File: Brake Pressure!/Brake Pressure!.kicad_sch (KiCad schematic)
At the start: 12 parts, among them J1 DTF13-6P, Q1 Q_Photo_NPN_EBC, U1 TJA1050DRG, U2 MCP2515-I, X1 ${ALTIUM_VALUE}

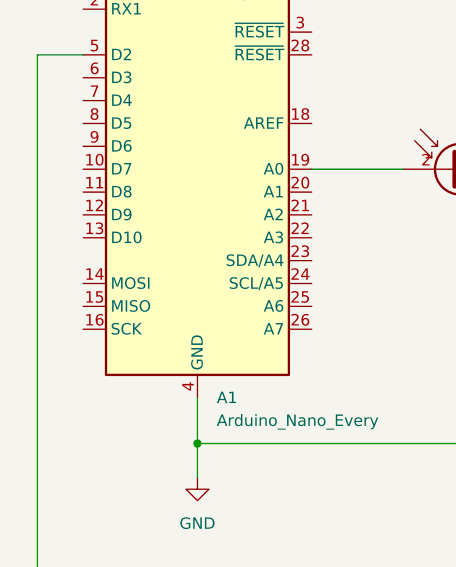
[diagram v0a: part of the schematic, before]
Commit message: make new connection
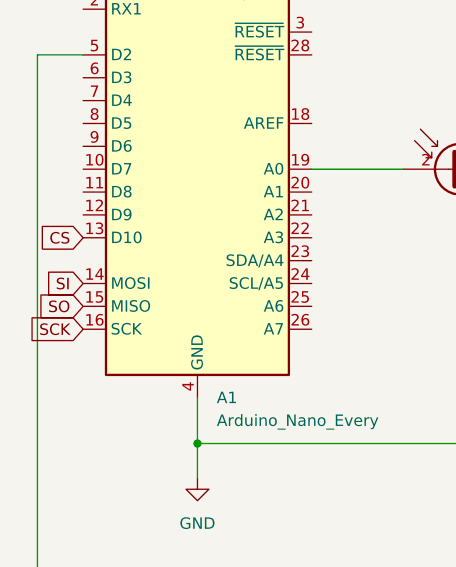
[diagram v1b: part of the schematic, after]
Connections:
- net CS: now also A1.13 (D10)
- net SCK: now also A1.16 (SCK)
- net SI: now also A1.14 (MOSI)
- net SO: now also A1.15 (MISO)
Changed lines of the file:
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@@
+		)
+	)
+	(global_label "SCK"
+		(shape input)
+		(at 30.48 68.58 180)
+		(fields_autoplaced yes)
+		(effects
+			(font
+				(size 1.27 1.27)
+			)
+			(justify right)
+		)
+		(property "Intersheetrefs" "${INTERSHEET_REFS}"
+			(at 23.7453 68.58 0)
+			(effects
+				(font
+					(size 1.27 1.27)
+				)
+				(justify right)
+				(hide yes)
+			)
 		)
 	)
@@
 		)
 	)
+	(global_label "CS"
+		(shape input)
+		(at 30.48 58.42 180)
+		(fields_autoplaced yes)
+		(effects
+			(font
+				(size 1.27 1.27)
+			)
+			(justify right)
+		)
+		(property "Intersheetrefs" "${INTERSHEET_REFS}"
+			(at 25.0153 58.42 0)
+			(effects
+				(font
+					(size 1.27 1.27)
+				)
+				(justify right)
+				(hide yes)
+			)
+		)
+	)
 	(global_label "Low"
 		(shape input)
@@
 		)
 	)
+	(global_label "SI"
+		(shape input)
+		(at 30.48 63.5 180)
+		(fields_autoplaced yes)
+		(effects
+			(font
+				(size 1.27 1.27)
+			)
+			(justify right)
+		)
+		(property "Intersheetrefs" "${INTERSHEET_REFS}"
+			(at 25.6805 63.5 0)
+			(effects
+				(font
+					(size 1.27 1.27)
+				)
+				(justify right)
+				(hide yes)
+			)
+		)
+	)
 	(global_label "SO"
 		(shape input)
@@
 				(hide yes)
 			)
+		)
+	)
+	(global_label "SO"
+		(shape input)
+		(at 30.48 66.04 180)
+		(fields_autoplaced yes)
+		(effects
+			(font
+				(size 1.27 1.27)
+			)
+			(justify right)
+		)
+		(property "Intersheetrefs" "${INTERSHEET_REFS}"
+			(at 24.9548 66.04 0)
+			(effects
+				(font
+					(size 1.27 1.27)
+				)
+				(justify right)
+				(hide yes)
+			)
